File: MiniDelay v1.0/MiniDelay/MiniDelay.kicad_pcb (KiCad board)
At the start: 2 copper layers, 45 x 128.5 mm, 53 parts, among them J1 IDC_2x05, U1 TL074, U2 PT2399

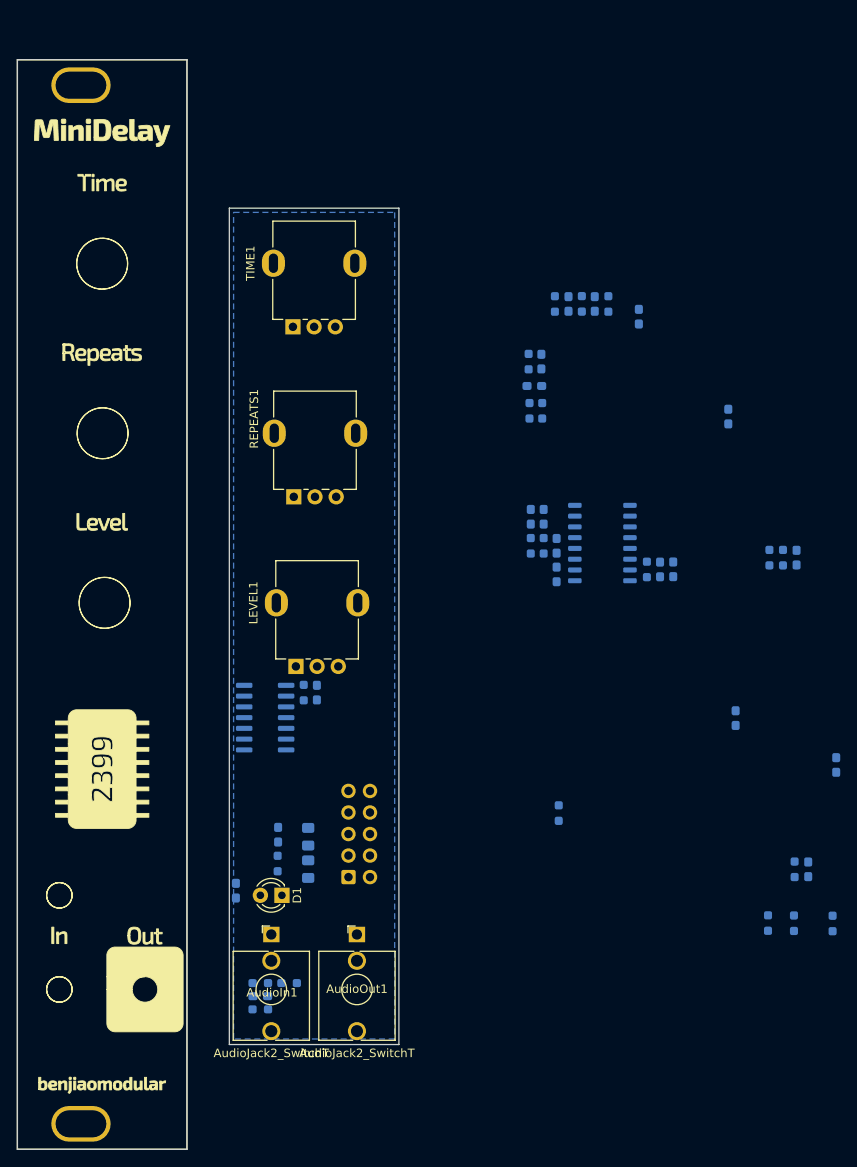
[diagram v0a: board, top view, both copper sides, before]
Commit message: Worked on BOM
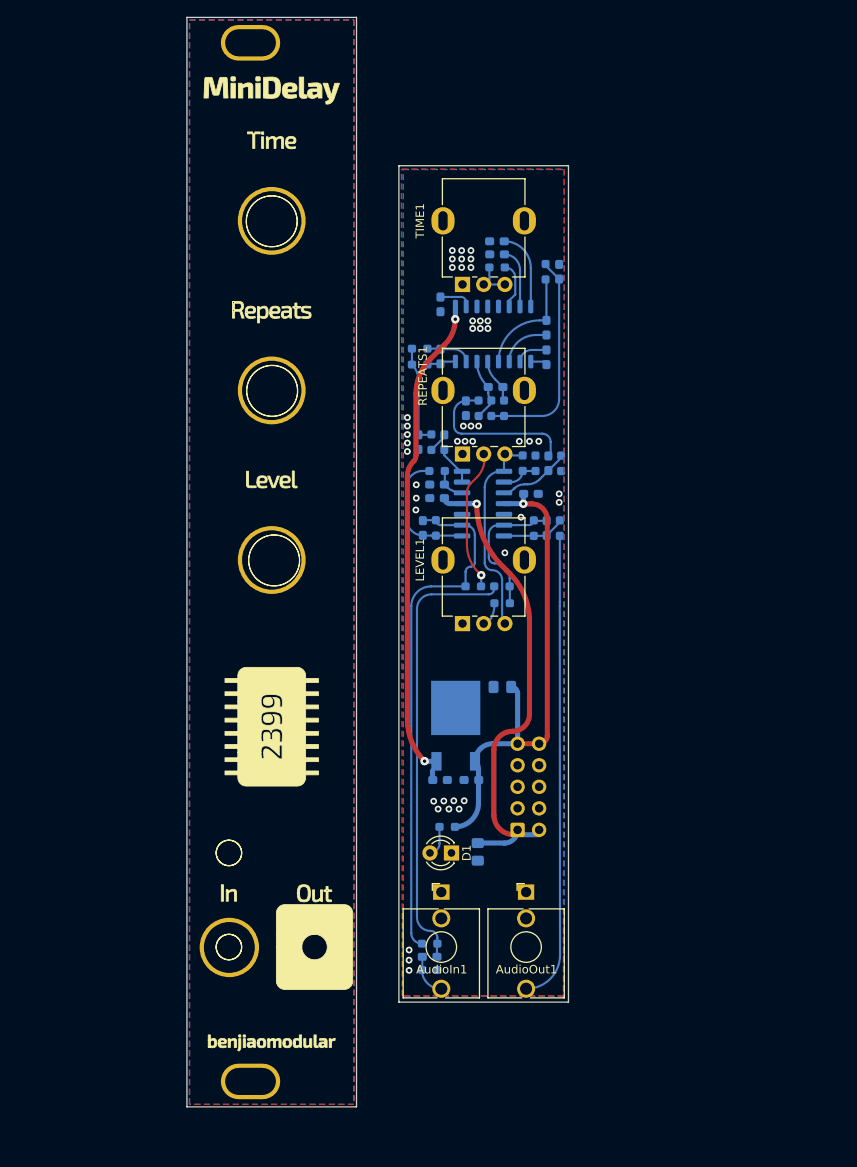
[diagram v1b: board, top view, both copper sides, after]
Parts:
- added REF**: PanelHole_Potentiometer_RV09, benjiaomodular:PanelHole_Potentiometer_RV09, F.Cu at (107.5, 91.5)
- added REF**: PanelHole_Potentiometer_RV09, benjiaomodular:PanelHole_Potentiometer_RV09, F.Cu at (107.5, 71.5)
- added REF**: PanelHole_AudioJack_3.5mm, benjiaomodular:PanelHole_AudioJack_3.5mm, F.Cu at (105.0, 143.2)
- added REF**: PanelHole_AudioJack_3.5mm, benjiaomodular:PanelHole_AudioJack_3.5mm, F.Cu at (115.0, 143.2)
- added REF**: PanelHole_Potentiometer_RV09, benjiaomodular:PanelHole_Potentiometer_RV09, F.Cu at (107.5, 111.5)
- added U3: L7805, Package_TO_SOT_SMD:TO-252-2, B.Cu at (131.7, 123.5)
- moved C7 71.6 mm to (129.9, 73.8)
- moved R11 63.1 mm to (129.5, 93.5), turned to 0 degrees
- moved C12 63.1 mm to (129.5, 95.1), turned to 0 degrees
- moved R9 56.7 mm to (144.0, 100.2)
- moved R6 51.6 mm to (133.8, 107.1)
- moved R18 51.1 mm to (137.2, 109.1), turned to 0 degrees
- moved R17 50.6 mm to (137.2, 107.1), turned to 0 degrees
- moved C9 43.9 mm to (136.6, 66.4), turned to 0 degrees
- moved C16 43.8 mm to (143.9, 70.0)
- moved R10 42.8 mm to (142.3, 70.0)
- moved C8 41.8 mm to (136.6, 67.9), turned to 0 degrees
- moved R16 41.3 mm to (144.1, 92.6), turned to 90 degrees
- moved R5 39.8 mm to (136.6, 69.5), turned to 180 degrees
- moved R8 37.3 mm to (137.4, 86.1)
- moved U1 36.0 mm to (134.9, 97.3)
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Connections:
- U1 pad 1: Net-(C6-Pad1) -> Net-(LEVEL1-Pad3)
- U1 pad 10: Net-(C21-Pad2) -> GND
- U1 pad 12: GND -> Net-(C12-Pad2)
- U1 pad 13: Net-(C22-Pad2) -> Net-(C18-Pad2)
- U1 pad 14: Net-(C22-Pad1) -> Net-(C18-Pad2)
- U1 pad 2: Net-(C6-Pad2) -> Net-(R19-Pad2)
- U1 pad 3: GND -> Net-(C21-Pad2)
- U1 pad 5: Net-(C12-Pad2) -> GND
- U1 pad 6: Net-(C18-Pad2) -> Net-(C22-Pad2)
- U1 pad 7: Net-(C18-Pad2) -> Net-(C22-Pad1)
- U1 pad 8: Net-(LEVEL1-Pad3) -> Net-(C6-Pad1)
- U1 pad 9: Net-(R19-Pad2) -> Net-(C6-Pad2)
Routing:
- net Net-(C6-Pad2): track 0.00 -> 61.9 mm
- net +12V: track 0.00 -> 58.8 mm, vias 0 -> 1
- net +5V: track 0.00 -> 58.3 mm, vias 0 -> 2
- net -12V: track 0.00 -> 56.9 mm, vias 0 -> 1
- net Net-(AudioOut1-PadT): track 0.00 -> 55.5 mm
- net DRY_OUT: track 0.00 -> 53.0 mm
- net Net-(LEVEL1-Pad3): track 0.00 -> 26.3 mm
- net Net-(C16-Pad2): track 0.00 -> 25.7 mm
- net Net-(C19-Pad2): track 0.00 -> 19.2 mm
- net Net-(C22-Pad2): track 0.00 -> 17.3 mm
- net REPEATS: track 0.00 -> 16.7 mm, vias 0 -> 1
- net Net-(C6-Pad1): track 0.00 -> 15.0 mm
- net Net-(C11-Pad2): track 0.00 -> 13.1 mm
- net Net-(C20-Pad1): track 0.00 -> 11.9 mm
- net Net-(C9-Pad2): track 0.00 -> 9.35 mm
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- added copper zone on B.Cu, net (none)
- added copper zone on F.Cu, net (none)
- added copper zone on F.Cu, net GND
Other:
- board text added: "MiniDelay v1.0"
- board text added: "by benjiaomodular"
